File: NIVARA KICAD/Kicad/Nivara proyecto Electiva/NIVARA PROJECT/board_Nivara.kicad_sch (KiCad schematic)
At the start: 6 parts, among them U2 ESP32-S3-WROOM-1

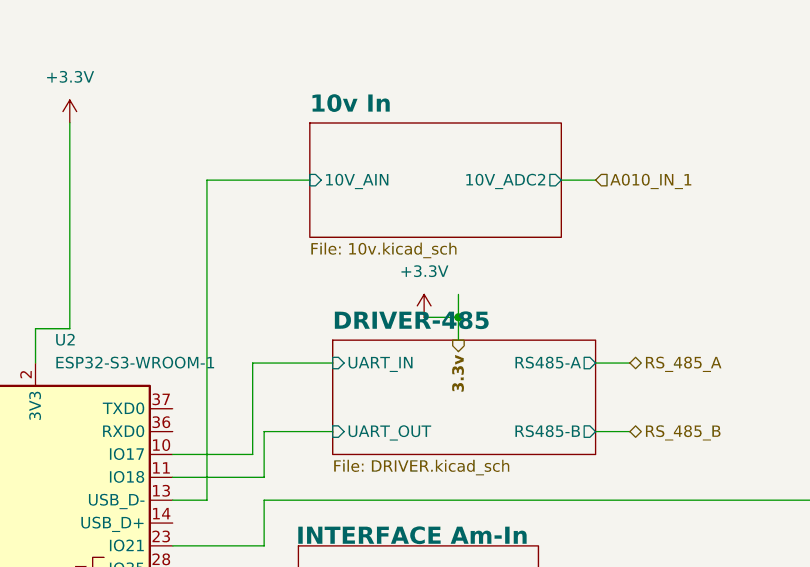
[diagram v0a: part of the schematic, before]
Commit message: Add files via upload
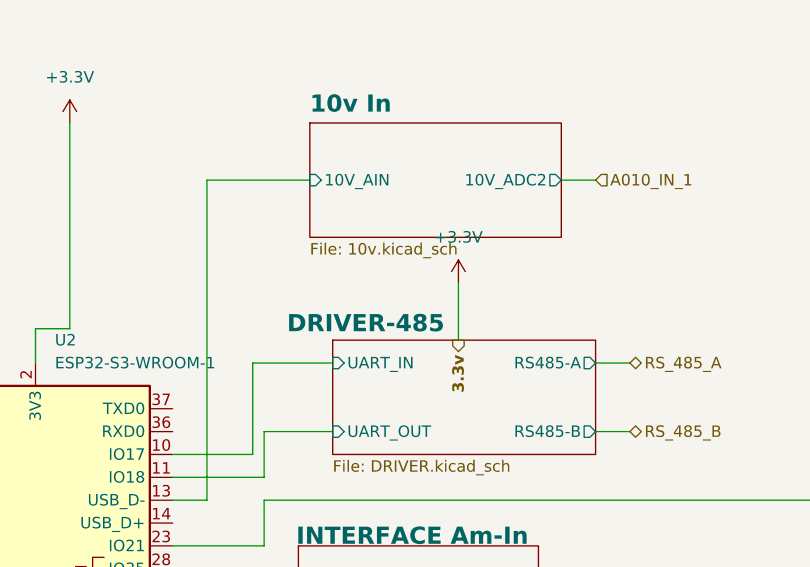
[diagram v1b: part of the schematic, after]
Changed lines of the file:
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@@
 		(color 0 0 0 0)
 	)
-	(junction
-		(at 191.77 45.72)
-		(diameter 0)
-		(color 0 0 0 0)
-	)
 	(wire
 		(pts
@@
 	(wire
 		(pts
-			(xy 191.77 45.72) (xy 187.96 45.72)
-		)
-		(stroke
-			(width 0)
-			(type default)
-		)
-	)
-	(wire
-		(pts
 			(xy 66.04 123.19) (xy 73.66 123.19)
 		)
@@
 	(wire
 		(pts
-			(xy 191.77 43.18) (xy 191.77 45.72)
+			(xy 191.77 41.91) (xy 191.77 48.26)
 		)
 		(stroke
@@
 	(wire
 		(pts
-			(xy 191.77 45.72) (xy 191.77 48.26)
-		)
-		(stroke
-			(width 0)
-			(type default)
-		)
-	)
-	(wire
-		(pts
 			(xy 113.03 35.56) (xy 127 35.56)
 		)
@@
 	(symbol
 		(lib_id "power:+3.3V")
-		(at 187.96 45.72 0)
+		(at 191.77 41.91 0)
 		(unit 1)
 		(exclude_from_sim no)
@@
 		(fields_autoplaced yes)
 		(property "Reference" "#PWR017"
-			(at 187.96 49.53 0)
+			(at 191.77 45.72 0)
 			(effects
 				(font
@@
 		)
 		(property "Value" "+3.3V"
-			(at 187.96 40.64 0)
+			(at 191.77 36.83 0)
 			(effects
 				(font
@@
 		)
 		(property "Footprint" ""
-			(at 187.96 45.72 0)
+			(at 191.77 41.91 0)
 			(effects
 				(font
@@
 		)
 		(property "Datasheet" ""
-			(at 187.96 45.72 0)
+			(at 191.77 41.91 0)
 			(effects
 				(font
@@
 		)
 		(property "Description" "Power symbol creates a global label with name \"+3.3V\""
-			(at 187.96 45.72 0)
+			(at 191.77 41.91 0)
 			(effects
 				(font
@@
 		(on_board yes)
 		(dnp no)
-		(fields_autoplaced yes)
 		(stroke
 			(width 0.1524)
@@
 		)
 		(property "Sheetname" "DRIVER-485"
-			(at 177.8 47.2309 0)
+			(at 172.72 47.498 0)
 			(effects
 				(font
